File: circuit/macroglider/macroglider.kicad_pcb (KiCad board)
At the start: 2 copper layers, 165 x 75 mm, 47 parts, among them SW1 Capacitive Button, SW2 Capacitive Button, SW3 Capacitive Button, SW4 Capacitive Button, SW5 Capacitive Button, SW6 Capacitive Button, SW7 Capacitive Button, SW8 Capacitive Button, SW9 Capacitive Button, U1 Pico

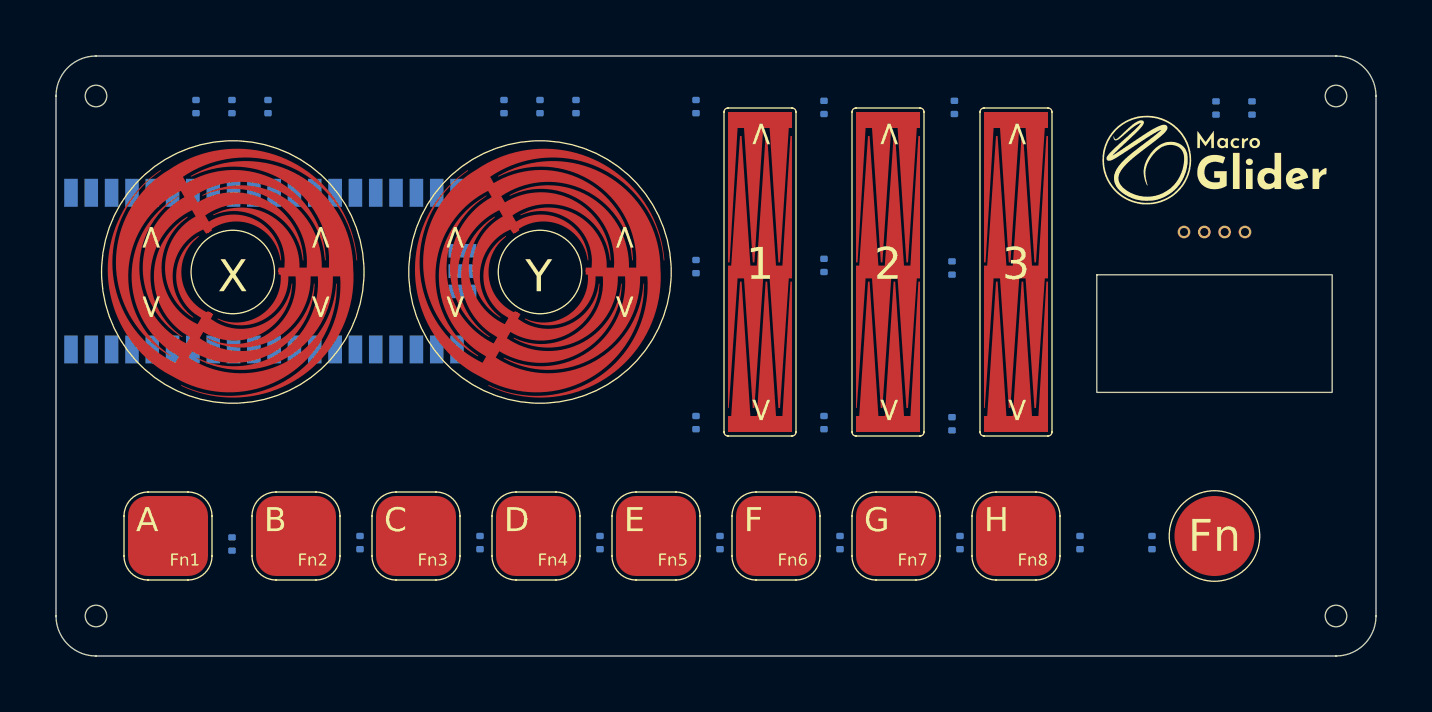
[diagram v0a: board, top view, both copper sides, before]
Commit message: changes
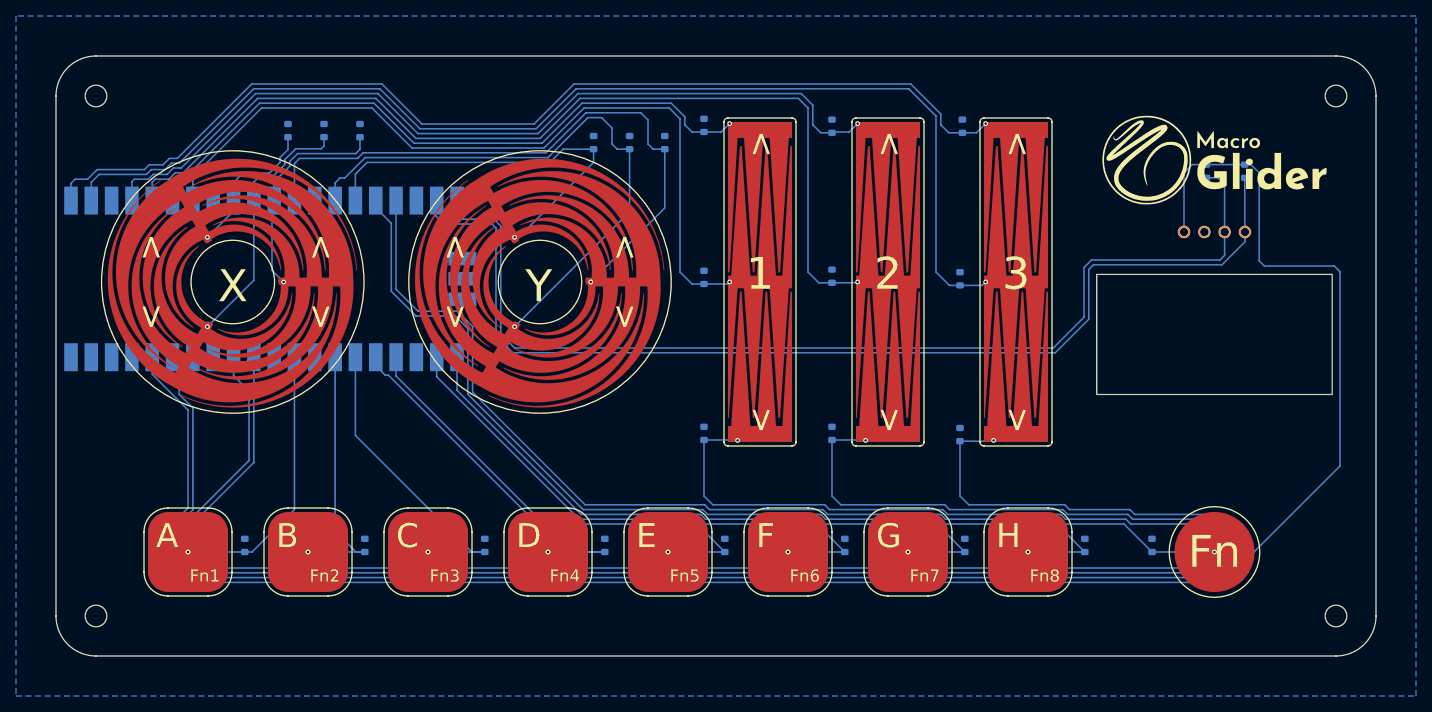
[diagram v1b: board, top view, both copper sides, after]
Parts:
- OLED1: footprint easyeda2kicad:OLED-TH_L35.4-W33.5_HS13L03W2C01 -> easyeda2kicad:OLED-TH_L35.4-W33.5_HS13L03W2C01_without_mount_outline
- moved R19 20.7 mm to (113.0, 64.3)
- moved R22 20.6 mm to (151.1, 65.8)
- moved R23 8.07 mm to (142.2, 65.8)
- moved R24 8.07 mm to (146.7, 65.8)
- moved R26 7.99 mm to (218.8, 69.4)
- moved R25 7.95 mm to (223.6, 69.4)
- moved R20 7.62 mm to (104.0, 64.3)
- moved R21 7.62 mm to (108.5, 64.3)
- moved SW1 3.20 mm to (91.5, 117.0)
- moved R13 2.55 mm to (172.0, 63.8)
- moved R16 2.55 mm to (188.3, 63.8)
- moved R10 2.55 mm to (156.0, 63.7)
- moved SW2 2.50 mm to (106.5, 117.0)
- moved SW3 2.50 mm to (121.5, 117.0)
- moved SW4 2.50 mm to (136.5, 117.0)
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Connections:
- U1 pad 1: /FADER1B -> /FADER3A
- U1 pad 10: /ROT1A -> /ROT1C
- U1 pad 11: /ROT1B -> /ROT1A
- U1 pad 12: /ROT1C -> /ROT2A
- U1 pad 14: /ROT2A -> /ROT2C
- U1 pad 16: /ROT2C -> /TPAD8
- U1 pad 2: /FADER2B -> /FADER3B
- U1 pad 31: /FADER3C -> /FADER1C
- U1 pad 34: /FADER1C -> /FADER3C
- U1 pad 4: /FADER3B -> /FADER2A
- U1 pad 5: /FADER3A -> /FADER2B
- U1 pad 7: /FADER2A -> /FADER1B
- U1 pad 9: /TPAD8 -> /ROT1B
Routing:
- net +3V3: track 0.00 -> 248.7 mm
- net /FADER1C: track 0.00 -> 244.4 mm, vias 0 -> 1
- net /FADER2C: track 0.00 -> 232.0 mm, vias 0 -> 1
- net /FADER3C: track 0.00 -> 216.5 mm, vias 0 -> 1
- net /FADER3B: track 0.00 -> 144.8 mm, vias 0 -> 1
- net /SDA: track 0.00 -> 135.5 mm
- net /SCL: track 0.00 -> 132.4 mm
- net /TPADFN: track 0.00 -> 131.9 mm, vias 0 -> 1
- net /FADER3A: track 0.00 -> 129.5 mm, vias 0 -> 1
- net /TPAD8: track 0.00 -> 124.3 mm, vias 0 -> 1
- net /FADER2B: track 0.00 -> 120.5 mm, vias 0 -> 1
- net /FADER2A: track 0.00 -> 105.6 mm, vias 0 -> 1
- net /FADER1B: track 0.00 -> 98.1 mm, vias 0 -> 1
- net /TPAD7: track 0.00 -> 84.0 mm, vias 0 -> 1
- net /FADER1A: track 0.00 -> 82.6 mm, vias 0 -> 1
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- added copper zone on B.Cu, net GND
